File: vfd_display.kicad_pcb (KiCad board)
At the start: 2 copper layers, 154 x 54 mm, 80 parts, among them J1 Conn_01x04, J2 Conn_01x04, J3 PJ-036AH-SMT-TR, Q1 STD16N65M5, U1 LR12LG-G, U2 AP62250WU-7, U3 GP1294AI, U4 LM3478, U5 AP62250WU-7

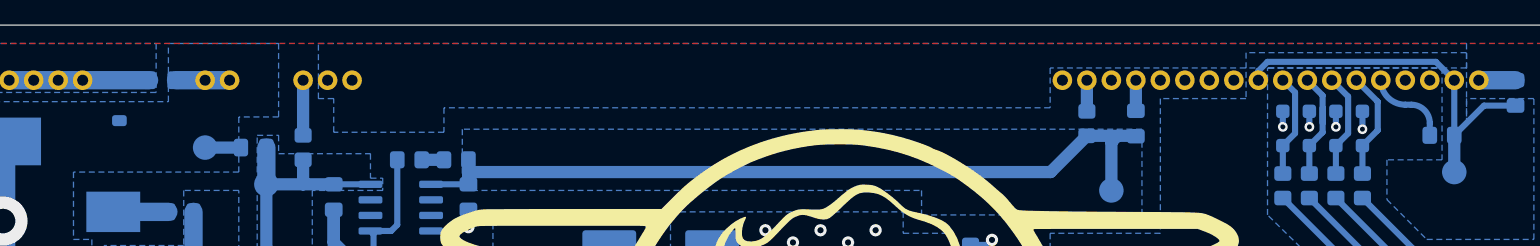
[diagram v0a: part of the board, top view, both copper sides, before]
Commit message: GP1278BI Variation
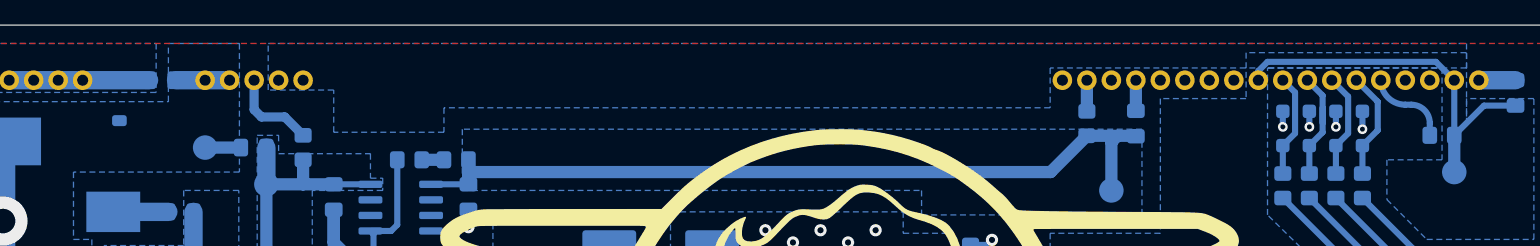
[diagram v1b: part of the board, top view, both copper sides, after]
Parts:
- U3: footprint Remi_Footprints:VFD_GP1294AI -> Remi_Footprints:VFD_GP1287BI
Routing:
- net Net-(U3-VHP): track 4.50 -> 7.27 mm
